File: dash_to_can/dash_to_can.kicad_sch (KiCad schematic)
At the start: 50 parts, among them J1 AVR-ISP1, J2 Conn_02x10_Top_Bottom, Q1 2N3904, Q10 AO3401A, Q2 2N3904, Q3 2N3904, Q4 AO3401A, Q5 2N3904, Q6 AO3401A, Q7 2N3904, Q8 AO3401A, Q9 2N3904, U1 ATmega328P-A, U2 LM7805_TO220, U3 MCP2515-xST, U4 TJA1050T_CM_118, U5 ULN2003A, U6 MCP41010, Y1 16MHz, Y2 Crystal

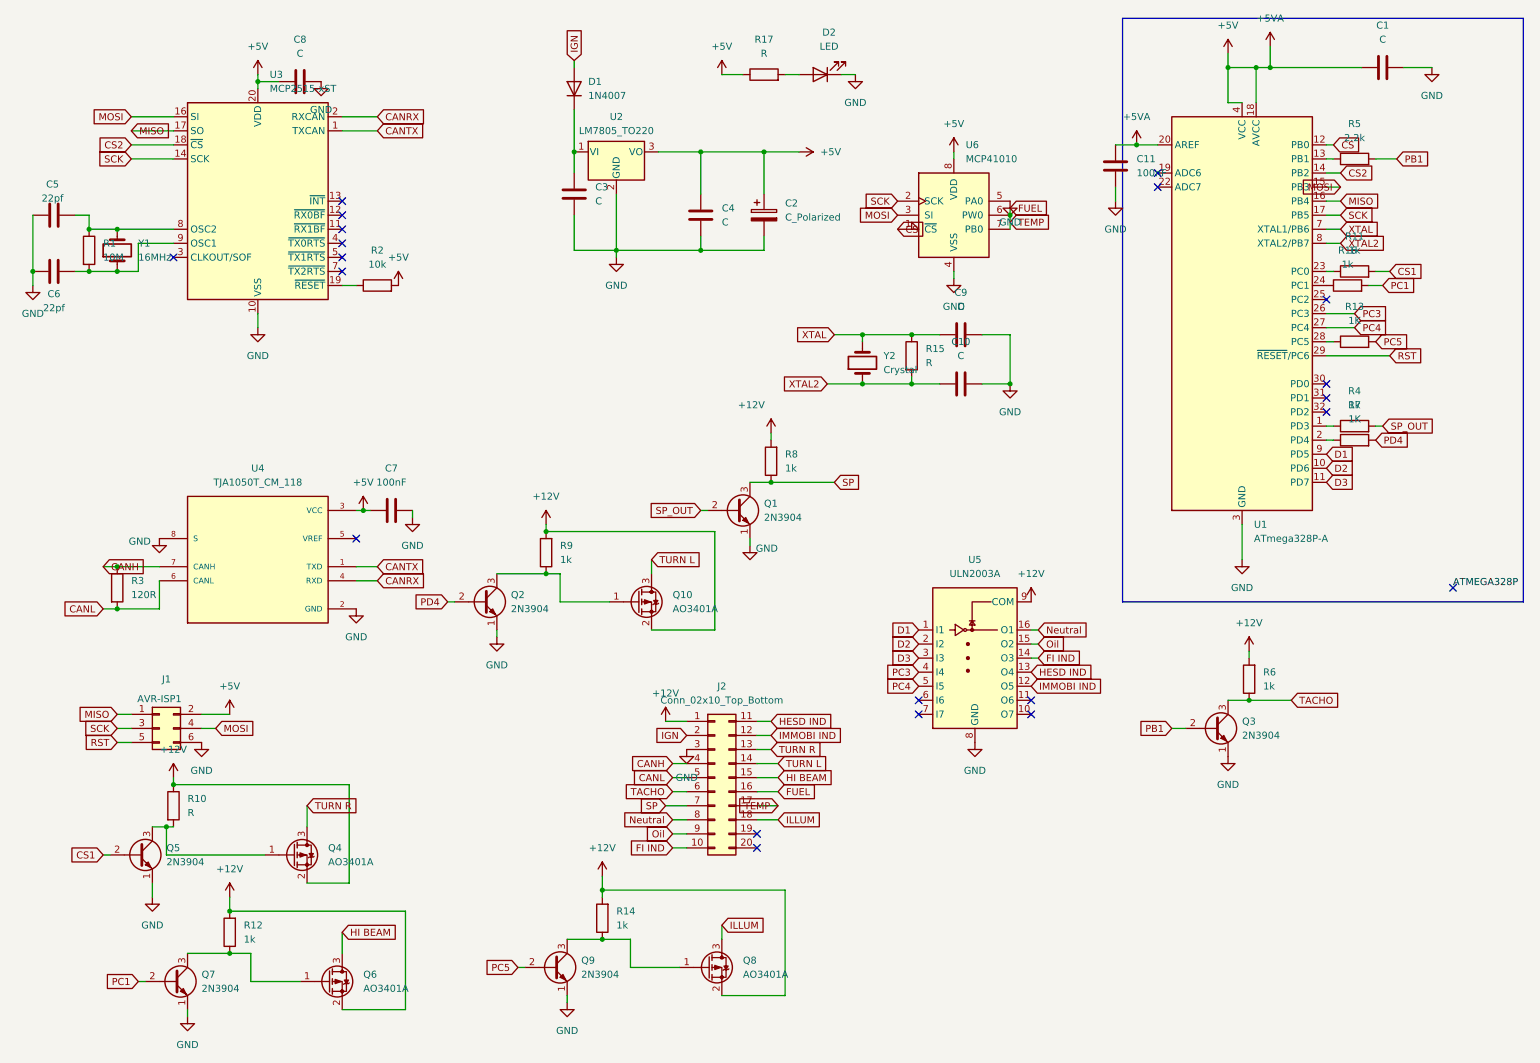
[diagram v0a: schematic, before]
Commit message: Uploading my (Gabriel's) changes
Tweaking and organising schematic
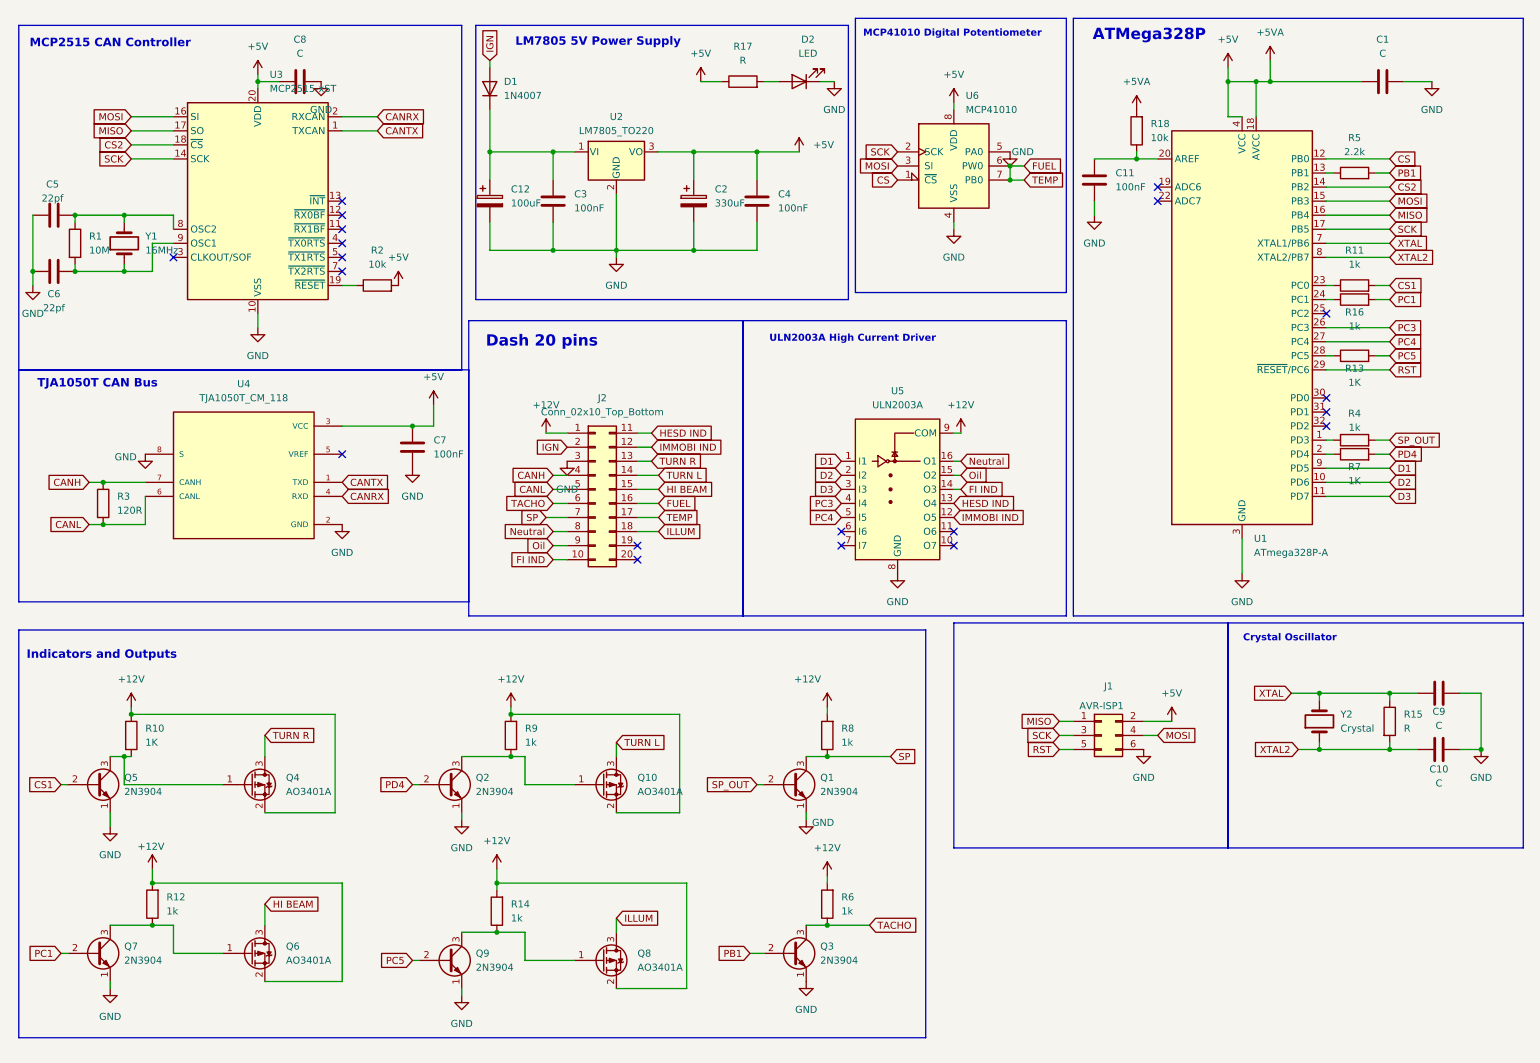
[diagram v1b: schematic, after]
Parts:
- added C12: 100uF, Capacitor_SMD:CP_Elec_4x3, symbol Device:C_Polarized
- added R18: 10k, Resistor_SMD:R_0201_0603Metric, symbol Device:R
- C2: value C_Polarized -> 330uF
- C3, C4: value C -> 100nF
- R10: value R -> 1K
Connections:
- net +5V: now also C7.2, R18.2; no longer C11.2, C7.1, U1.20 (AREF)
- net GND: now also C7.1, C12.2; no longer C7.2
- net at C3.1, D1.1 (K), U2.1 (VI): now also C12.1
- new net: C11.2, R18.1, U1.20 (AREF)
- no-connect marks 21 -> 20
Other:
- note added: "ATMega328P"
- note added: "Crystal Oscillator"
- note added: "Dash 20 pins"
- note added: "Indicators and Outputs"
- note added: "LM7805 5V Power Supply"
- note added: "MCP2515 CAN Controller"
- note added: "MCP41010 Digital Potentiometer"
- note added: "TJA1050T CAN Bus"
- note added: "ULN2003A High Current Driver"
- moved on the sheet: C1, C10, C11, C2, C3, C4, C7, C9, D1, D2, J1, J2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
